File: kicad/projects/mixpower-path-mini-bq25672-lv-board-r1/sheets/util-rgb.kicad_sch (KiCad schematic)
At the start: 7 parts, among them Q5 PJE8405, U7 SN74LV1T125DCK

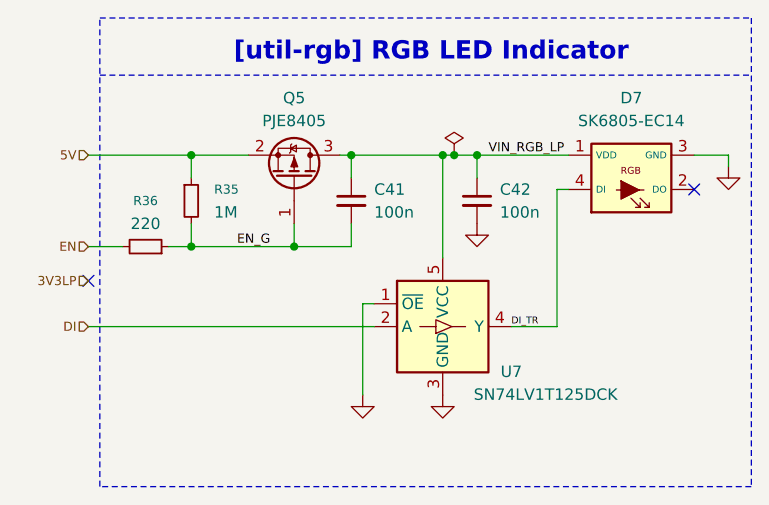
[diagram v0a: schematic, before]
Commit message: feat: failed PCB routing
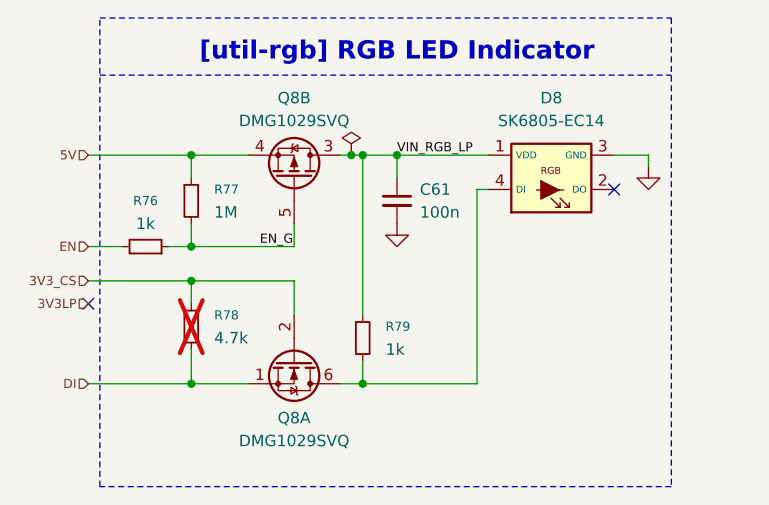
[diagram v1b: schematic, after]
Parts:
- removed C41: 100n, Capacitor_SMD:C_0402_1005Metric, symbol Device:C_Small
- removed Q5: PJE8405, mixlib-generic-sot:SOT-523, symbol mixlib-discrete-mosfet:PJE8405
- removed U7: SN74LV1T125DCK, Package_TO_SOT_SMD:SOT-353_SC-70-5, symbol Logic_LevelTranslator:SN74LV1T125DCK
- added Q8: DMG1029SVQ, mixlib-generic-sot:SOT-563, symbol mixlib-discrete-mosfet:DMG1029SVQ
- added R78: 4.7k, Resistor_SMD:R_0402_1005Metric, symbol Device:R_Small
- added R79: 1k, Resistor_SMD:R_0402_1005Metric, symbol Device:R_Small
- R76: renamed from R36; value 220 -> 1k
- renumbered C42 to C61, D7 to D8, R35 to R77
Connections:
- net 5V: now also Q8.4 (S2)
- net DI: now also Q8.1 (S1), R78.2
- net EN_G: now also Q8.5 (G2)
- net VIN_RGB_LP: now also Q8.3 (D2), R79.1
- net DI_TR: no longer names the net of D8.4 (DI)
- net DI_TR: now also Q8.6 (D1), R79.2
- new net 3V3_CS: Q8.2 (G1), R78.1
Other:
- moved on the sheet: C61, D8
